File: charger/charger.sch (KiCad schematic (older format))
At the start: 105 parts, among them J1 OSTT7020150, J2 Conn_01x06, J3 Conn_01x06, J4 Conn_01x03, J5 OSTT7020150, Q1 CSD18540Q5B, Q2 CSD19531Q5A, Q3 CSD19531Q5A, Q4 CSD19531Q5A, Q5 CSD19531Q5A, Q6 CSD18540Q5B, U1 MSP432, U2 NCP718xSN500, U3 UCC27517DBVR, U4 INA240A2PW, U5 LM5109BMA, U6 LM5109BMA, U7 INA240A2PW, U8 LM5009MM, U9 AP131-33

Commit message: finished pcb
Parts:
- R24: footprint Resistor_SMD:R_1206_3216Metric -> Resistor_SMD:R_2512_6332Metric
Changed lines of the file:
@@
 F 0 "R24" V 8045 2500 50  0000 C CNN
 F 1 "0.002" V 8136 2500 50  0000 C CNN
-F 2 "Resistor_SMD:R_1206_3216Metric" V 8290 2490 50  0001 C CNN
-F 3 "~" H 8250 2500 50  0001 C CNN
+F 2 "Resistor_SMD:R_2512_6332Metric" V 8290 2490 50  0001 C CNN
+F 3 "https://www.mouser.com/ProductDetail/Yageo/PU2512FKMP50R002L?qs=sGAEpiMZZMvdGkrng054t0c0U24Fa%2Fv2NfStLNxNcuIQTzdklHgYjw%3D%3D" H 8250 2500 50  0001 C CNN
 	1    8250 2500
 	0    1    1    0

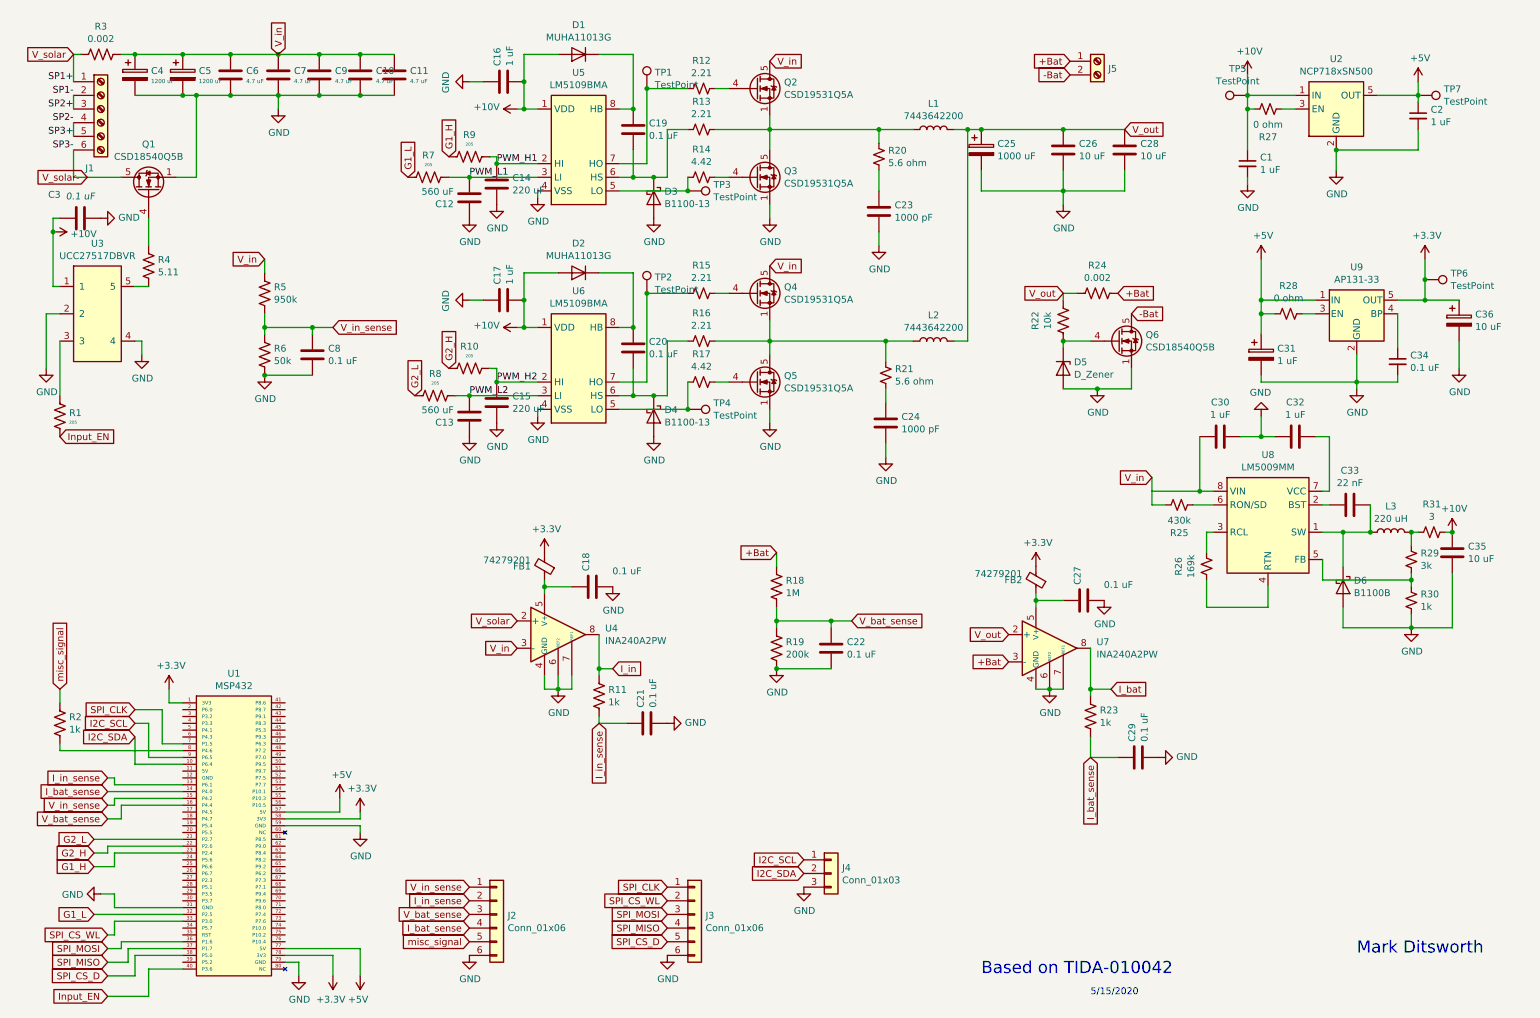
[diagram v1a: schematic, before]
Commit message: charger pcb v2
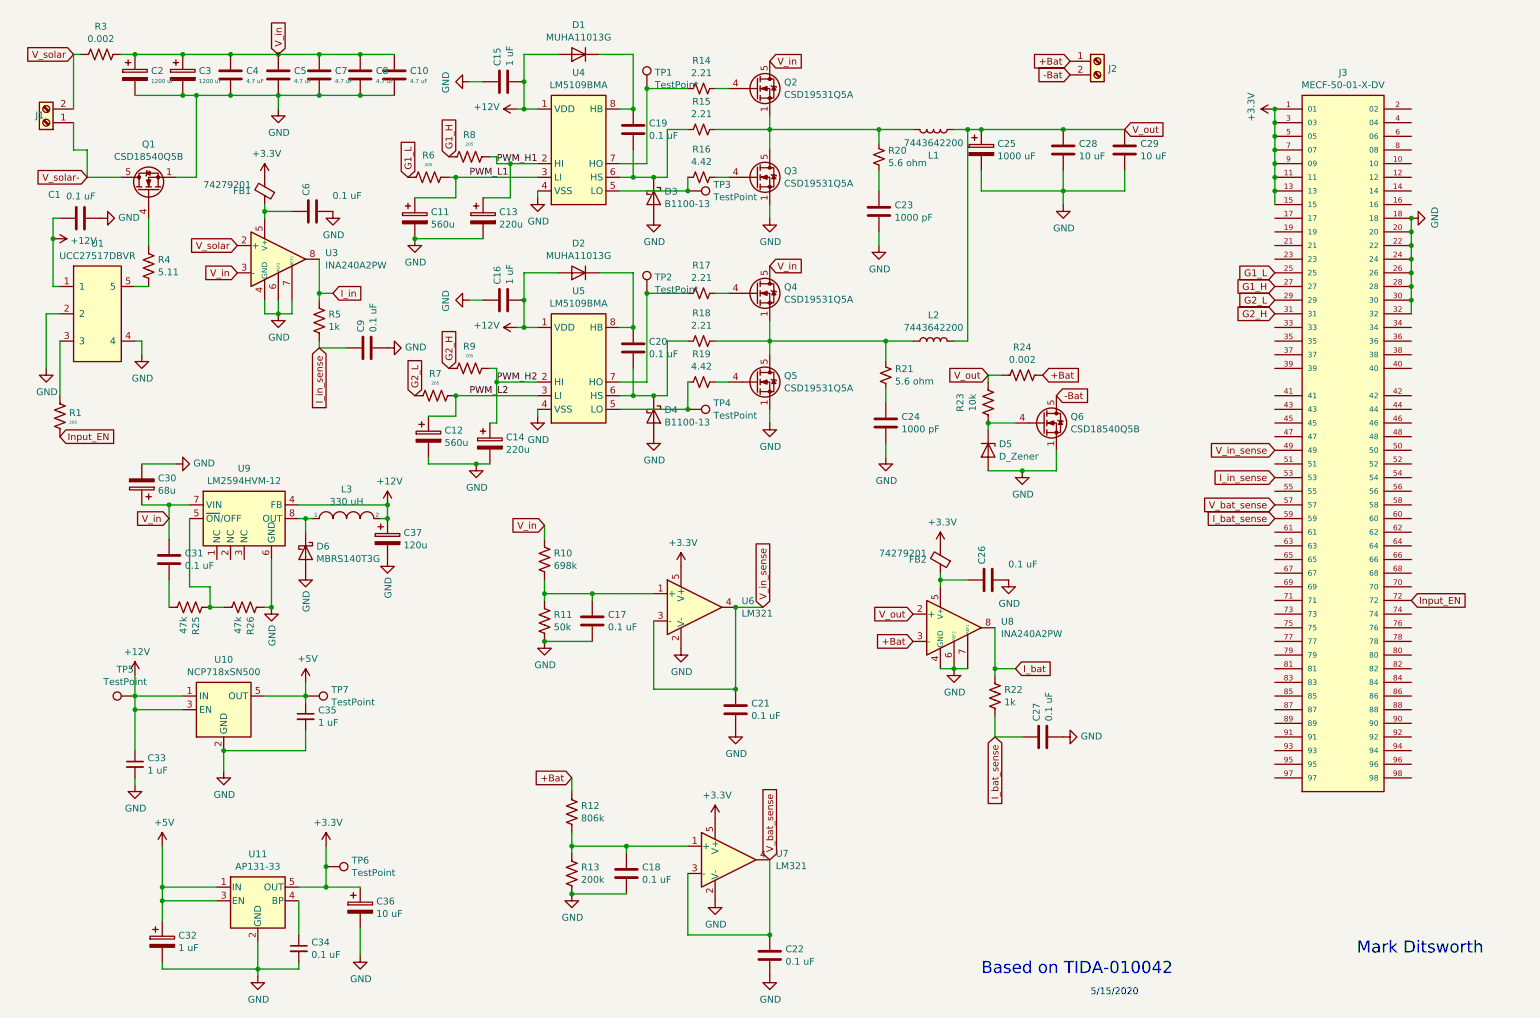
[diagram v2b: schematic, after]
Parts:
- removed C12, C13: 560 uF, Capacitor_SMD:C_1206_3216Metric, symbol Device:C
- removed C14, C15: 220 uF, Capacitor_SMD:C_1206_3216Metric, symbol Device:C
- removed C30, C32: 1 uF, Capacitor_SMD:C_1206_3216Metric, symbol Device:C
- removed C33: 22 nF, Capacitor_SMD:C_1206_3216Metric, symbol Device:C
- removed C35: 10 uF, Capacitor_SMD:C_1206_3216Metric, symbol Device:C
- removed D6: B1100B, Diode_SMD:D_SMB, symbol Device:D_Schottky
- removed J1: OSTT7020150, Connector_PinHeader_2.54mm:PinHeader_1x06_P2.54mm_Vertical, symbol Connector:Screw_Terminal_01x06
- removed J2, J3: Conn_01x06, Connector_PinHeader_2.54mm:PinHeader_1x06_P2.54mm_Vertical, symbol Connector_Generic:Conn_01x06
- removed J4: Conn_01x03, Connector_PinHeader_2.54mm:PinHeader_1x03_P2.54mm_Vertical, symbol Connector_Generic:Conn_01x03
- removed L3: 220 uH, Inductor_SMD:L_Bourns_SRR1260, symbol Device:L
- removed R2: 1k, Resistor_SMD:R_1206_3216Metric, symbol Device:R_US
- removed R25: 430k, Resistor_SMD:R_1206_3216Metric, symbol Device:R_Small_US
- removed R26: 169k, Resistor_SMD:R_1206_3216Metric, symbol Device:R_Small_US
- removed R27, R28: 0 ohm, Resistor_SMD:R_1206_3216Metric, symbol Device:R_Small_US
- removed R29: 3k, Resistor_SMD:R_1206_3216Metric, symbol Device:R_Small_US
- removed R30: 1k, Resistor_SMD:R_1206_3216Metric, symbol Device:R_Small_US
- removed R31: 3, Resistor_SMD:R_1206_3216Metric, symbol Device:R_Small_US
- removed U1: MSP432, MWD_Footprints:MSP432, symbol MSP_mwd:MSP432
- removed U8: LM5009MM, Package_SO:MSOP-8_3x3mm_P0.65mm, symbol Regulator_Switching:LM5009MM
- added C11, C12: 560u, Capacitor_SMD:C_Elec_8x10.2, symbol Device:CP
- added C13, C14: 220u, Capacitor_SMD:C_Elec_6.3x7.7, symbol Device:CP
- added C21, C22, C31: 0.1 uF, Capacitor_SMD:C_1206_3216Metric, symbol Device:C
- added C30: 68u, Capacitor_SMD:C_Elec_8x10.2, symbol Device:CP
- added C37: 120u, Capacitor_SMD:C_Elec_10x10.2, symbol Device:CP
- added D6: MBRS140T3G, Diode_SMD:D_SMB_Handsoldering, symbol Diode:1N5819
- added J1: OSTT7020150, MWD_Footprints:Phoenix_MKDS_6.35, symbol Connector:Screw_Terminal_01x02
- added J3: MECF-50-01-X-DV, SAMTEC_MECF-50-01-X-DV, symbol MECF-50-01-X-DV:MECF-50-01-X-DV
- added L3: 330 uH, Inductor_SMD:L_Bourns_SRR1260, symbol pspice:INDUCTOR
- added R25, R26: 47k, Resistor_SMD:R_1206_3216Metric, symbol Device:R_US
- added U6, U7: LM321, Package_TO_SOT_SMD:SOT-23-5, symbol Amplifier_Operational:LM321
- added U9: LM2594HVM-12, Package_SO:SOIC-8_3.9x4.9mm_P1.27mm, symbol Regulator_Switching:LM2594HVM-12
- J2: renamed from J5; footprint Connector_PinHeader_2.54mm:PinHeader_1x02_P2.54mm_Vertical -> MWD_Footprints:Phoenix_MKDS_6.35
- R10: renamed from R5; value 950k -> 698k
- R12: renamed from R18; value 1M -> 806k
- R3: footprint Resistor_SMD:R_1206_3216Metric -> Resistor_SMD:R_2512_6332Metric
- U3: renamed from U4; footprint Package_SO:TSSOP-8_4.4x3mm_P0.65mm -> Package_SO:SOIC-8_3.9x4.9mm_P1.27mm
- U8: renamed from U7; footprint Package_SO:TSSOP-8_4.4x3mm_P0.65mm -> Package_SO:SOIC-8_3.9x4.9mm_P1.27mm
- renumbered C3 to C1, C11 to C10, C16 to C15, C17 to C16, C8 to C17, C22 to C18, C4 to C2, C27 to C26, C29 to C27, C26 to C28, C28 to C29, C5 to C3, C31 to C32, C1 to C33, C2 to C35, C6 to C4, C7 to C5, C18 to C6, C9 to C7, C10 to C8, C21 to C9, R6 to R11, R19 to R13, R12 to R14, R13 to R15, R14 to R16, R15 to R17, R16 to R18, R17 to R19, R23 to R22, R22 to R23, R11 to R5, R7 to R6, R8 to R7, R9 to R8, R10 to R9, U3 to U1, U2 to U10, U9 to U11, U5 to U4, U6 to U5
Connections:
- net +10V is gone; now on net +12V: C1.2, C15.2, C16.2, C33.1, D1.2 (A), D2.2 (A), TP5.1, U1.1, U10.1 (IN), U4.1 (VDD), U5.1 (VDD)
- net +3V3: now also J3.1 (01), J3.11, J3.13, J3.15, J3.3 (03), J3.5 (05), J3.7 (07), J3.9 (09), U6.5 (V+), U7.5 (V+)
- net +5V: now also U11.3 (EN)
- net G1_H: now also J3.27
- net G1_L: now also J3.25
- net G2_H: now also J3.31
- net G2_L: now also J3.29
- net GND: now also C11.2, C12.2, C13.2, C14.2, C21.2, C22.2, C30.2, C37.2, D6.2 (A), J3.18, J3.20, J3.22, J3.24, J3.26, J3.28, J3.30, J3.32, R26.1, U6.2 (V-), U7.2 (V-), U9.6 (GND)
- net I_bat_sense: now also J3.59
- net I_in_sense: now also J3.53
- net Input_EN: now also J3.72
- net PWM_H1: now also C13.1
- net PWM_H2: now also C14.1
- net PWM_L1: now also C11.1
- net PWM_L2: now also C12.1
- net V_bat_sense: now also C22.1, J3.57, U7.3 (-), U7.4; no longer C18.1, R12.2, R13.1
- net V_in: now also C30.1, C31.1, U9.7 (VIN)
- net V_in_sense: now also C21.1, J3.49, U6.3 (-), U6.4; no longer C17.1, R10.2, R11.1
- net V_out: now also L1.1; no longer L1.2
- net V_solar: now also J1.2 (Pin_2)
- net V_solar-: now also J1.1 (Pin_1)
- net +12V: now reaches U10.3 (EN)
- net +12V: now also C37.1, L3.2, U9.4 (FB)
- net at Q2.1 (S), Q2.2 (S), Q2.3 (S)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: now also L1.2; no longer L1.1
- new net: C17.1, R10.2, R11.1, U6.1 (+)
- new net: C18.1, R12.2, R13.1, U7.1 (+)
- new net: R25.1, R26.2, U9.5 (~ON~/OFF)
- new net: D6.1 (K), L3.1, U9.8 (OUT)
- new net: C31.2, R25.2
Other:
- moved on the sheet: C17, C18, C26, C27, C32, C33, C34, C35, C36, C6, C9, D5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
